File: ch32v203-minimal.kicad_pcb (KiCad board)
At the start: 2 copper layers, 50 x 30 mm, 21 parts, among them J1 Conn_01x08, J3 Conn_01x04, J4 Conn_01x04, J5 Conn_02x10_Odd_Even, SW1 SW_Push, SW2 SW_Push, U1 AMS1117-3.3, U2 CH32V203K8T6, Y1 8MHz

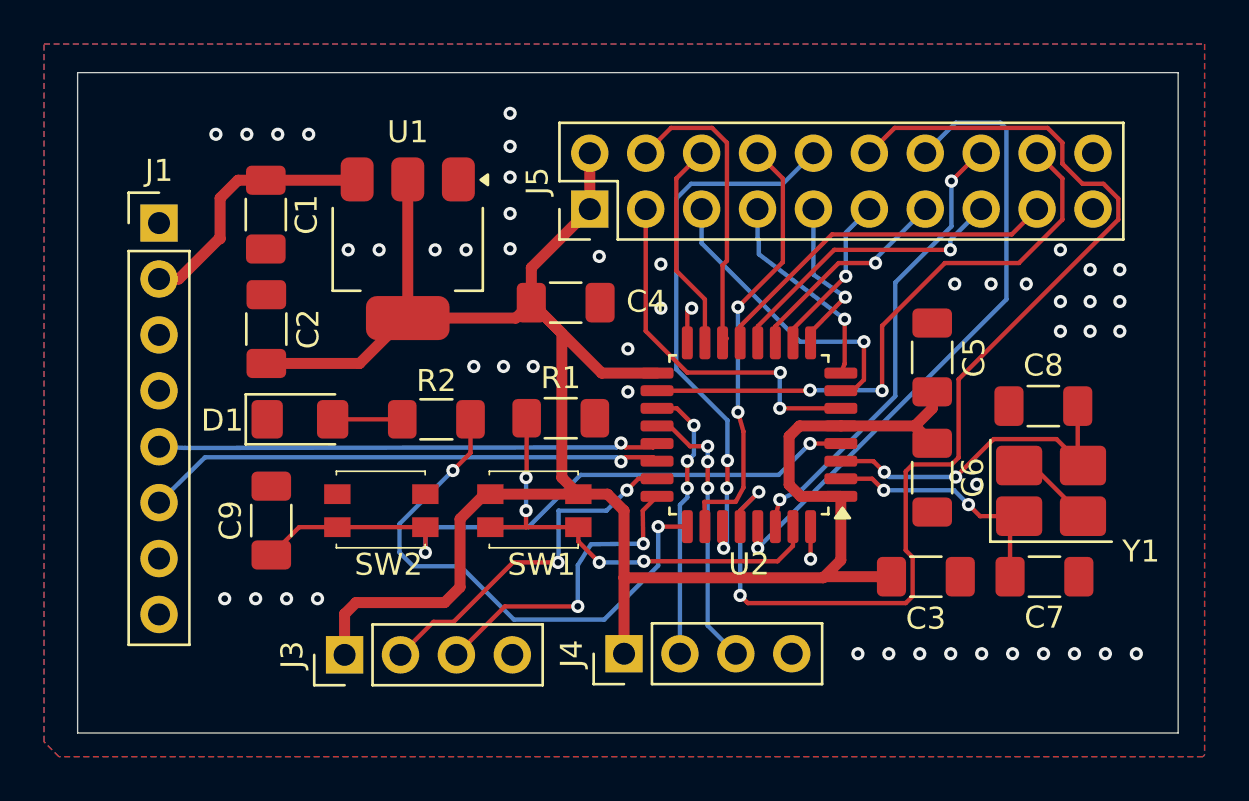
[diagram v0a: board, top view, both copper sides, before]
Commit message: Rework layout
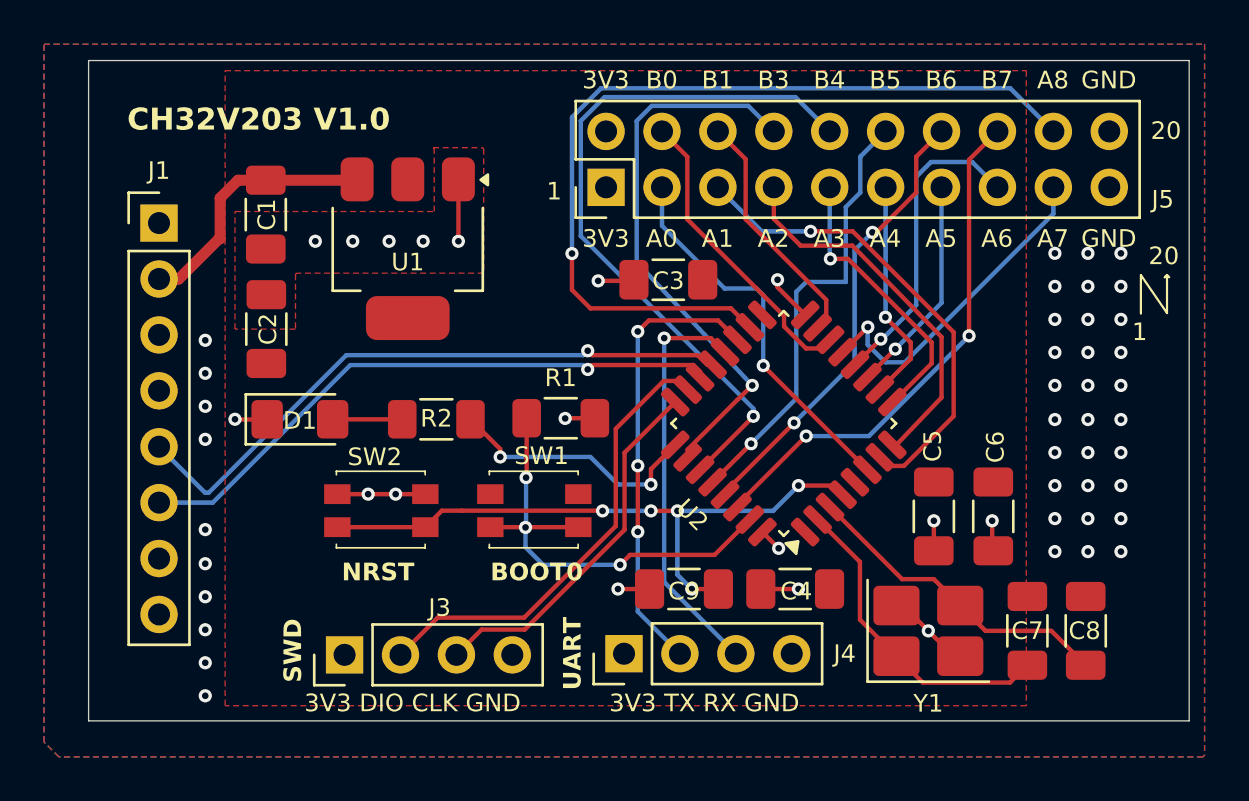
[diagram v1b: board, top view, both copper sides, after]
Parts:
- moved C9 19.0 mm to (158.2, 106.2), turned to 180 degrees
- moved C3 17.9 mm to (157.5, 92.1), turned to 180 degrees
- moved C4 16.7 mm to (163.2, 106.2), turned to 180 degrees
- moved C8 10.4 mm to (176.4, 108.1), turned to -90 degrees
- moved Y1 8.46 mm to (169.3, 108.1)
- moved C5 7.22 mm to (169.6, 102.9), turned to -90 degrees
- moved C6 3.29 mm to (172.2, 102.9)
- moved C7 2.58 mm to (173.8, 108.1), turned to -90 degrees
- moved U2 1.66 mm to (162.7, 98.6), turned to 135 degrees
- moved J5 1.24 mm to (154.7, 87.9)
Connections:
- net Net-(U2-BOOT0/PB8) renamed /BOOT0
- net Net-(U2-NRST) renamed /NRST
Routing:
- net +3V3: track 99.2 -> 0.02 mm
- net PB5: track 52.0 -> 20.3 mm, vias 2 -> 1
- net GND: track 7.03 -> 24.7 mm, vias 50 -> 57
- net PA8: track 26.9 -> 39.9 mm, vias 2 -> 1
- net Net-(U2-PA15): track 24.5 -> 11.9 mm
- net PB6: track 29.1 -> 20.7 mm, vias 1 -> 2
- net PA1: track 13.8 -> 21.7 mm
- net MCU_TX: track 12.6 -> 20.5 mm
- net PA2: track 9.45 -> 17.2 mm, vias 1 -> 0
- net PB4: track 25.0 -> 32.5 mm, vias 3 -> 1
- net /D-: track 22.9 -> 28.9 mm
- net MCU_RX: track 12.6 -> 18.7 mm, vias 3 -> 1
- net PB3: track 19.8 -> 25.6 mm, vias 2 -> 1
- net PA3: track 7.47 -> 12.9 mm
- net /SWDIO: track 16.3 -> 21.0 mm, vias 2 -> 0
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- added copper zone on F.Cu, net +3V3
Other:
- board text added: "1"
- board text added: "1 3 5 7 9 11 13 15 17 19"
- board text added: "10"
- board text added: "11"
- board text added: "12"
- board text added: "13"
- board text added: "14"
- board text added: "15"
- board text added: "16"
- board text added: "17"
- board text added: "18"
- board text added: "19"
- board text added: "2"
- board text added: "2 4 6 8 10 12 14 16 18 20"
- board text added: "20"
- board text added: "3"
- board text added: "3V3"
- board text added: "3V3 DIO CLK GND"
- board text added: "3V3 PA0 PA1 PA2 PA3 PA4 PA5 PA6 PA7 GND"
- board text added: "3V3 PB0 PB1 PB3 PB4 PB5 PB6 PB7 PA8 GND"
- board text added: "3V3 TX RX GND"
- board text added: "4"
- board text added: "5"
- board text added: "6"
- board text added: "7"
- board text added: "8"
- board text added: "9"
- board text added: "A0"
- board text added: "A1"
- board text added: "A2"
- board text added: "A3"
- board text added: "A4"
- board text added: "A5"
- board text added: "A6"
- board text added: "A7"
- board text added: "A8"
- board text added: "B0"
- board text added: "B1"
- board text added: "B3"
- board text added: "B4"
- board text added: "B5"
- board text added: "B6"
- board text added: "B7"
- board text added: "BOOT0"
- board text added: "CH32V203 V1.0"
- board text added: "GND"
- board text added: "NRST"
- board text added: "SWD"
- board text added: "UART"
